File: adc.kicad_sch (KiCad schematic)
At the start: 0 parts

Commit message: Lotta stuff added
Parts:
- added C10, C11: 1 uF, symbol Device:C
- added J: Pressure Sensor I/O, symbol Connector:Screw_Terminal_01x03
- added MC1: ~, symbol MC74A5-33SNTR:MC74A5-33SNTR
- added R10, R11, R12, R13, R14, R15, R6, R7, R8, R9: 10k, symbol Device:R
- added R16, R17: 3.3k, symbol Device:R
- added U1, U2: ADS1115IDGSR, ADS1115IDGSR:SOP50P490X110-10N, symbol ADS1115:ADS1115IDGSR
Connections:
- new net +3.3V: C10.1, C11.1, MC1.3 (VDD), R16.1, R17.1, R8.1, U1.8 (VDD), U2.1 (ADDR), U2.8 (VDD)
- new net +3.3V_meas: R8.2, R9.1, U1.4 (AIN0)
- new net +5V_meas: R10.2, R11.1, U1.5 (AIN1)
- new net +5v: J.1 (Pin_1), R10.1
- new net 12v(1)_Shutdown: R12.1
- new net 12v(1)_meas: R12.2, R13.1, U2.4 (AIN0)
- new net 12v(2)_Shutdown: R14.1
- new net 12v(2)_meas: R14.2, R15.1, U2.5 (AIN1)
- new net BAT+: R6.1
- new net BAT+_meas: R6.2, R7.1, U1.6 (AIN2)
- new net GND: C10.2, C11.2, J.3 (Pin_3), MC1.2 (GND), R11.2, R13.2, R15.2, R7.2, R9.2, U1.1 (ADDR), U1.3 (GND), U2.3 (GND)
- new net I2C_Bus1_SCL: MC1.4 (SCL), R17.2, U1.10 (SCL), U2.10 (SCL)
- new net I2C_Bus1_SDA: MC1.5 (SDA), R16.2, U1.9 (SDA), U2.9 (SDA)
- new net PS_Analog_V: J.2 (Pin_2), U1.7 (AIN3)
- no-connect marks 0 -> 3
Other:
- note added: "Analog - Digital Converters (ADCs)"
- note added: "Pressure Sensor"
- note added: "Slave Address: 1001000"
- note added: "Slave Address: 1001001"
- note added: "Temperature Sensor"
- note added: "Voltage Ladders: V_measure = 1/2 * V_actual"

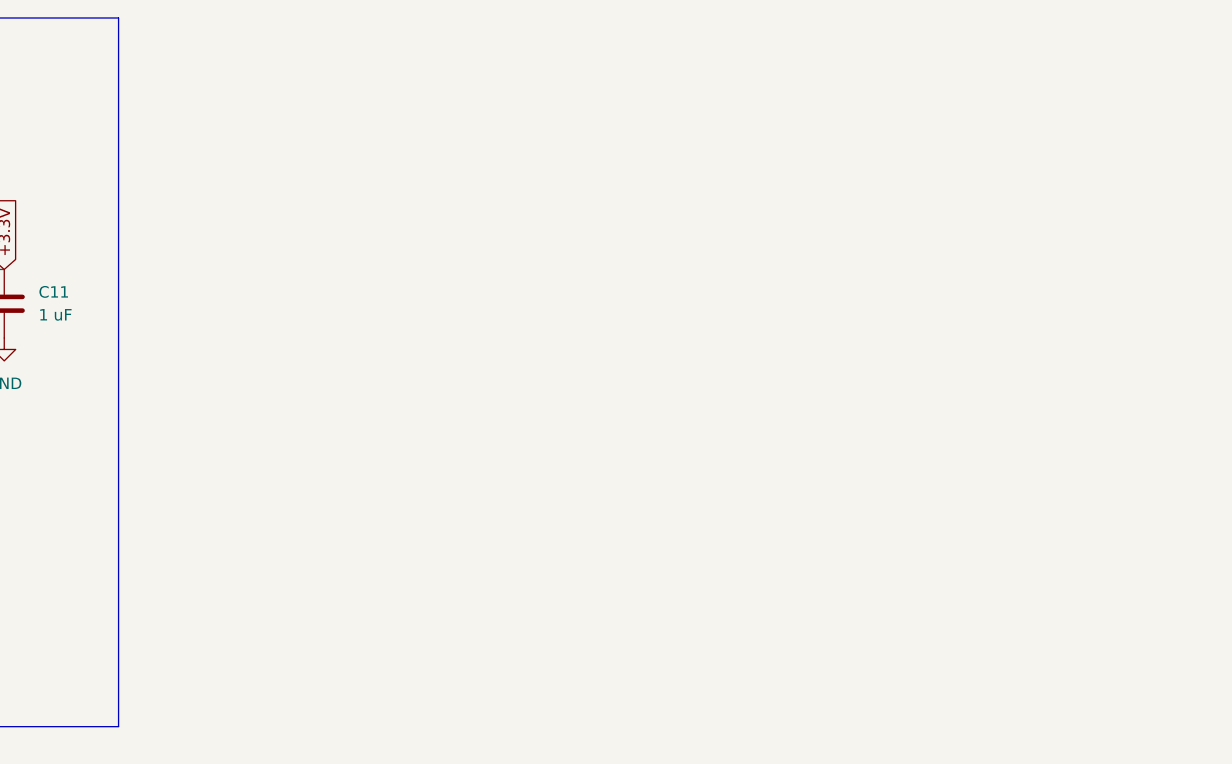
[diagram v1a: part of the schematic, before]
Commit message: routing
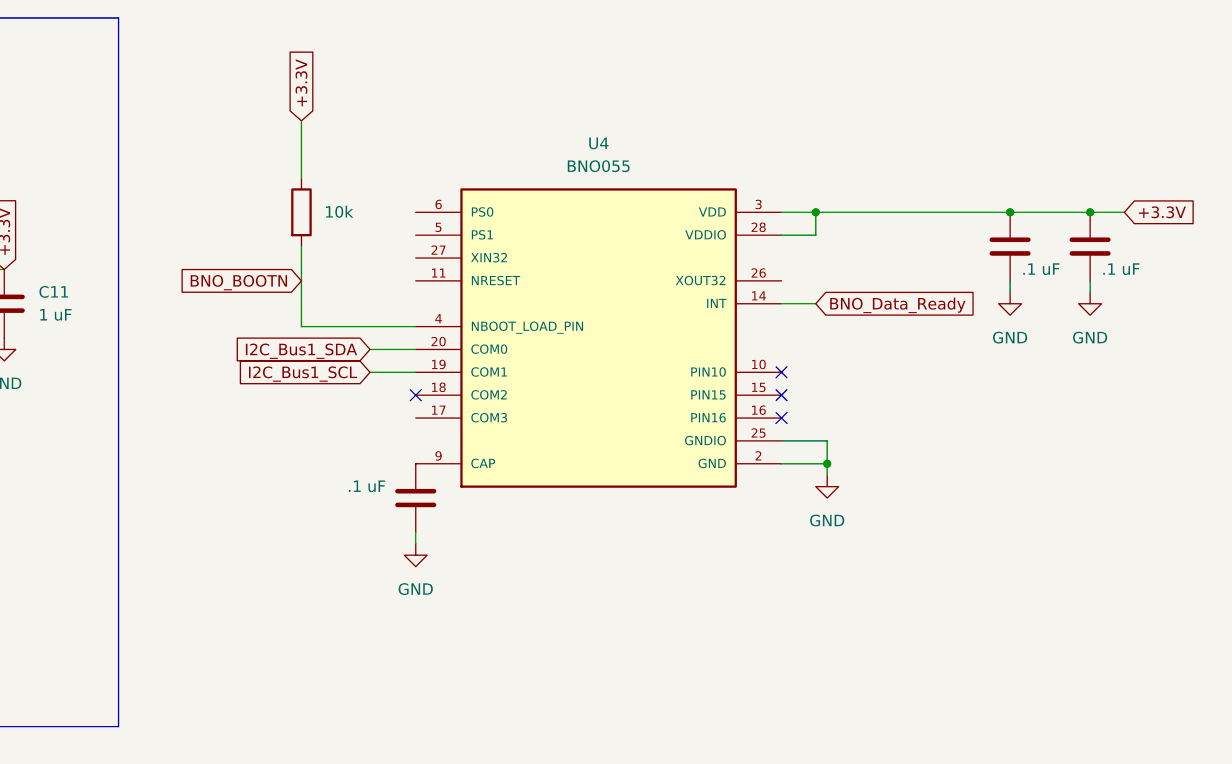
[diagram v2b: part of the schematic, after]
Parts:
- added C27, C28, C29: .1 uF, Capacitor_SMD:C_0603_1608Metric_Pad1.08x0.95mm_HandSolder, symbol Device:C
- added R18: 10k, Resistor_SMD:R_0603_1608Metric_Pad0.98x0.95mm_HandSolder, symbol Device:R
- added U4: BNO055, BNO055:LGA28R50P4X10_380X520X100, symbol BNO055:BNO055
- C10, C11: footprint (none) -> Capacitor_SMD:C_0603_1608Metric_Pad1.08x0.95mm_HandSolder
- J5: renamed from J; footprint (none) -> Connector_PinHeader_2.54mm:PinHeader_1x03_P2.54mm_Vertical_SMD_Pin1Right
- MC1: footprint (none) -> Package_TO_SOT_SMD:SOT-23-5_HandSoldering
- R10, R11, R12, R13, R14, R15, R16, R17, R6, R7, R8, R9: footprint (none) -> Resistor_SMD:R_0603_1608Metric_Pad0.98x0.95mm_HandSolder
- U1, U2: footprint ADS1115IDGSR:SOP50P490X110-10N -> ADS1115:SOP50P490X110-10N
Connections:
- net +3.3V: now also C27.1, C28.1, R18.1, U4.28 (VDDIO), U4.3 (VDD)
- net GND: now also C27.2, C28.2, C29.2, U4.2 (GND), U4.25 (GNDIO)
- net I2C_Bus1_SCL: now also U4.19 (COM1)
- net I2C_Bus1_SDA: now also U4.20 (COM0)
- new net: C29.1, U4.9 (CAP)
- new net BNO_BOOTN: R18.2, U4.4 (NBOOT_LOAD_PIN)
- new net BNO_Data_Ready: U4.14 (INT)
- no-connect marks 3 -> 7
